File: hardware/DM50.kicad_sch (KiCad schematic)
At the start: 99 parts, among them J1 ST-LINK, J2 USB_C_Receptacle_USB2.0_14P, Q1 MMBT3904, SW1 SW_SPST, SW10 BT_SMD, SW11 BT_SMD, SW12 BT_SMD, SW13 BT_SMD, SW14 BT_SMD, SW15 BT_SMD, SW16 BT_SMD, SW17 BT_SMD, SW18 BT_SMD, SW19 BT_SMD, SW2 BT_SMD, SW20 BT_SMD, SW21 BT_SMD, SW22 BT_SMD, SW23 BT_SMD, SW24 BT_SMD, SW25 BT_SMD, SW26 BT_SMD, SW27 BT_SMD, SW28 BT_SMD, SW29 BT_SMD, SW3 BT_SMD, SW30 BT_SMD, SW31 BT_SMD, SW32 BT_SMD, SW33 BT_SMD, SW34 BT_SMD, SW35 BT_SMD, SW36 BT_SMD, SW37 BT_SMD, SW38 BT_SMD, SW39 BT_SMD, SW4 BT_SMD, SW40 BT_SMD, SW41 BT_SMD, SW42 SW_SPST, SW43 BT_SMD, SW44 BT_SMD, SW45 BT_SMD, SW46 BT_SMD, SW47 BT_SMD, SW48 BT_SMD, SW49 BT_SMD, SW5 BT_SMD, SW50 BT_SMD, SW51 BT_SMD, SW52 BT_SMD, SW6 BT_SMD, SW7 BT_SMD, SW8 BT_SMD, SW9 BT_SMD, U1 EA_DOGL128X-6, U2 STM32U535CBT6, U3 AT25SF641, U4 USBLC6-2SC6, U5 ADP2108AUJ-3.3, Y1 32768

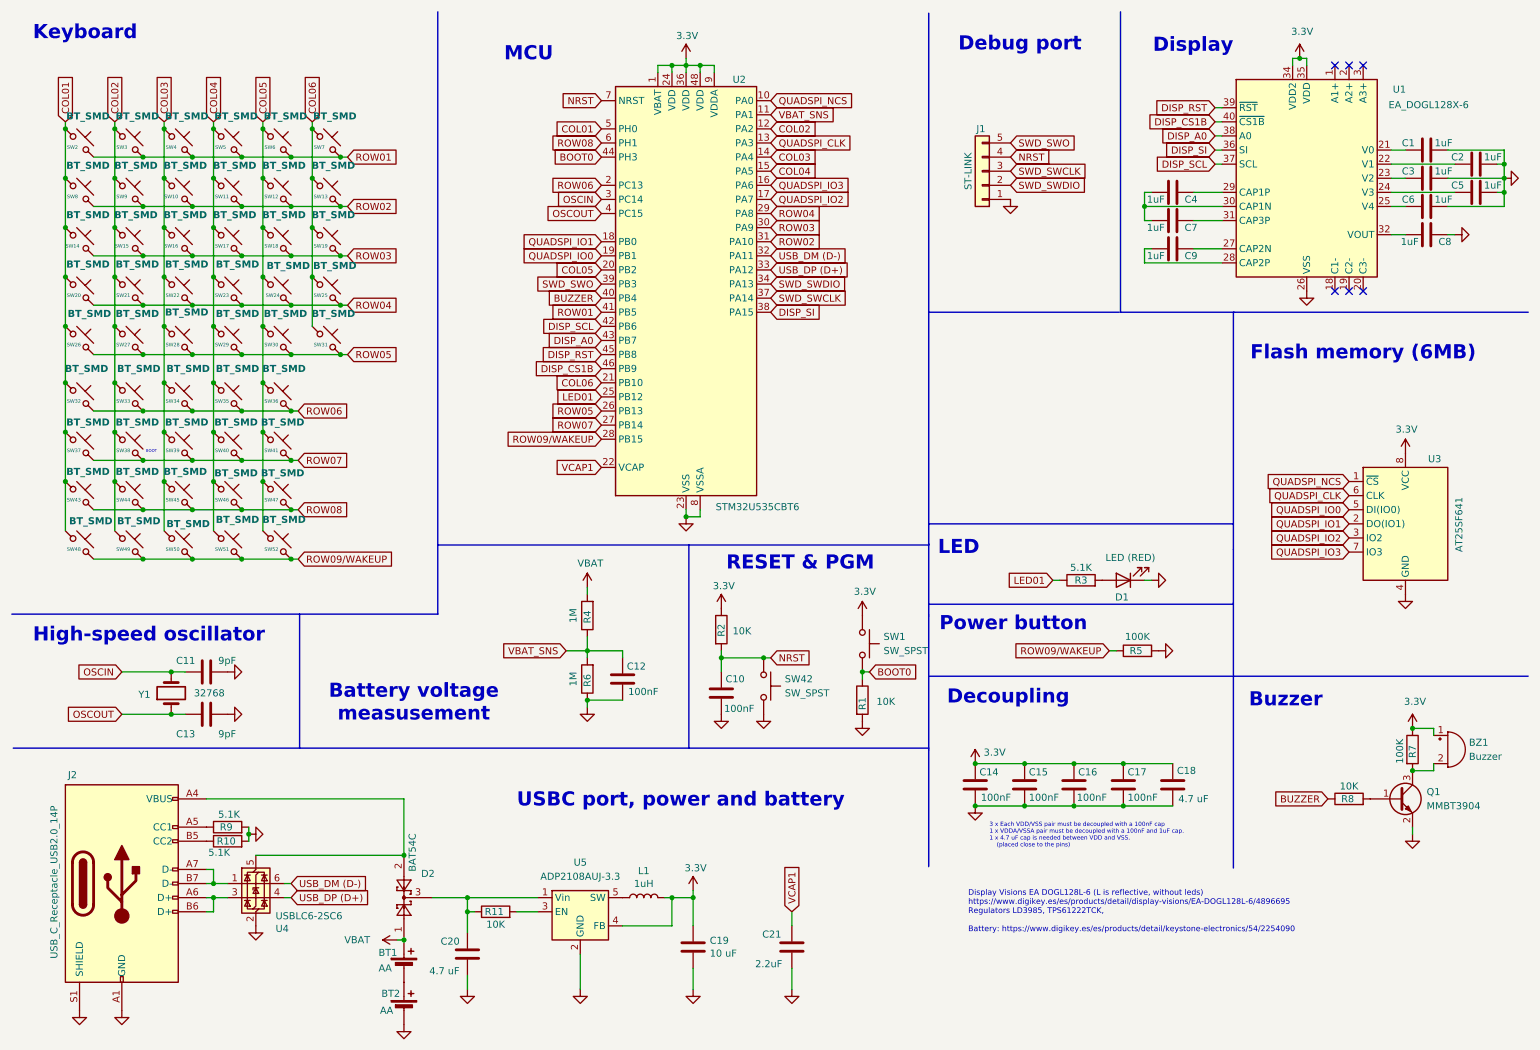
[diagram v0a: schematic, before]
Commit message: pcb changes
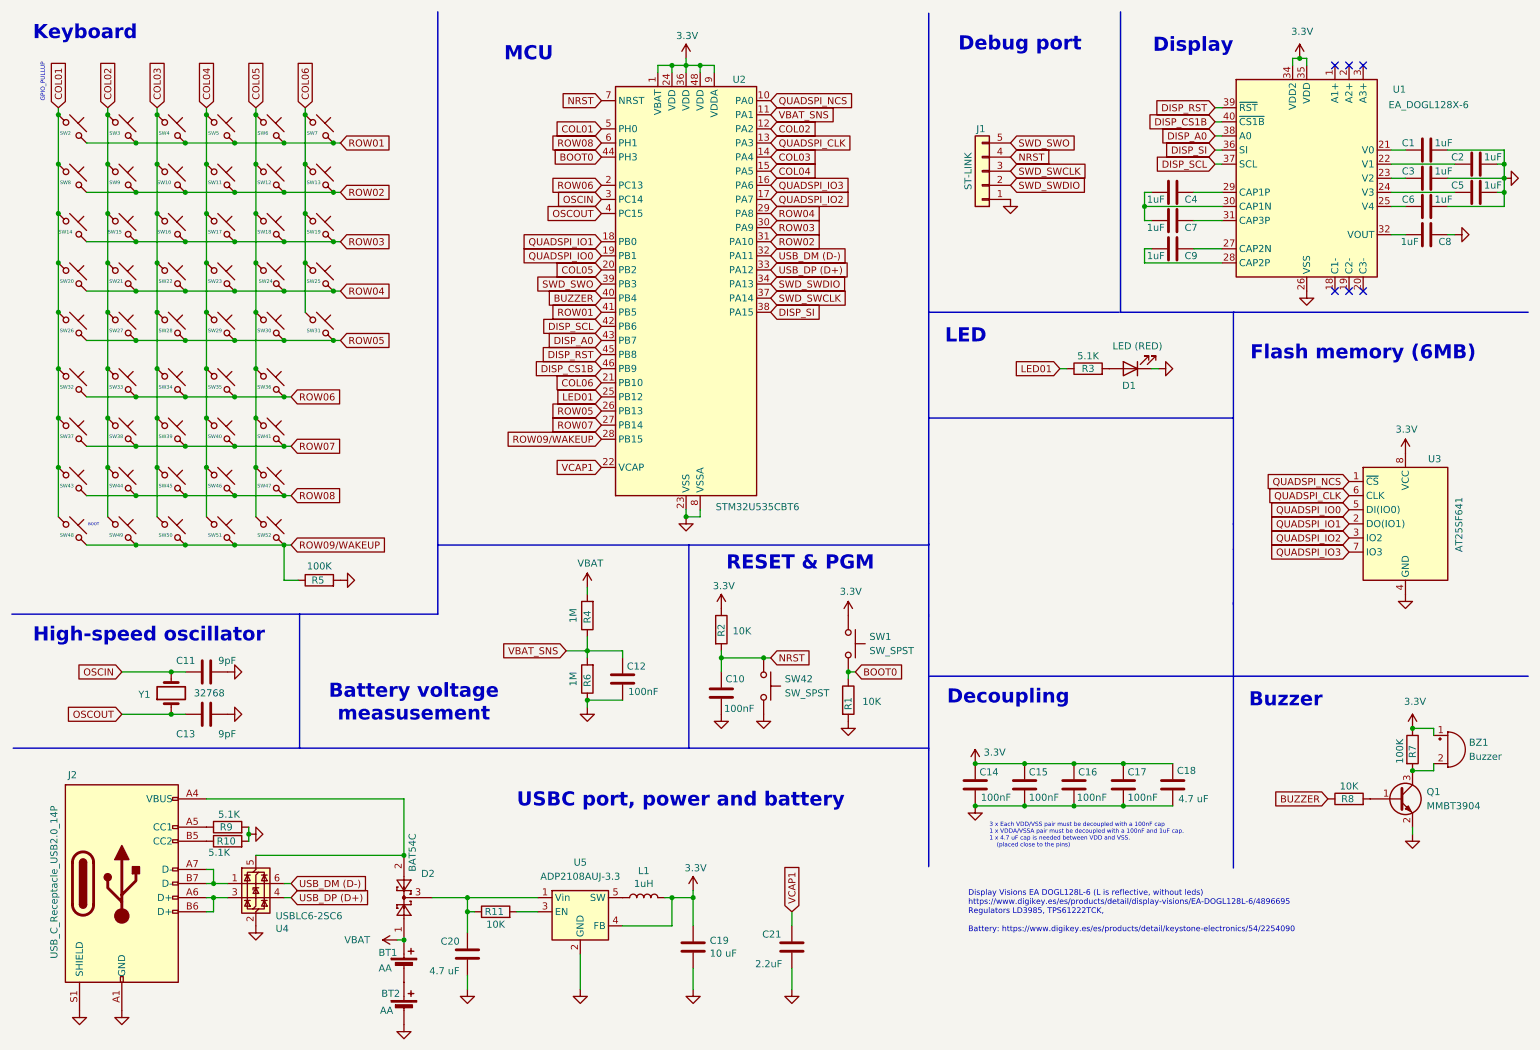
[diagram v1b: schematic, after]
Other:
- note added: "GPIO_PULLUP"
- note removed: "Power button"
- moved on the sheet: D1, R1, R3, R5, SW1, SW10, SW11, SW12, SW13, SW14, SW15, SW16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
